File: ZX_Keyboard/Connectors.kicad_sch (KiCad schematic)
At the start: 18 parts

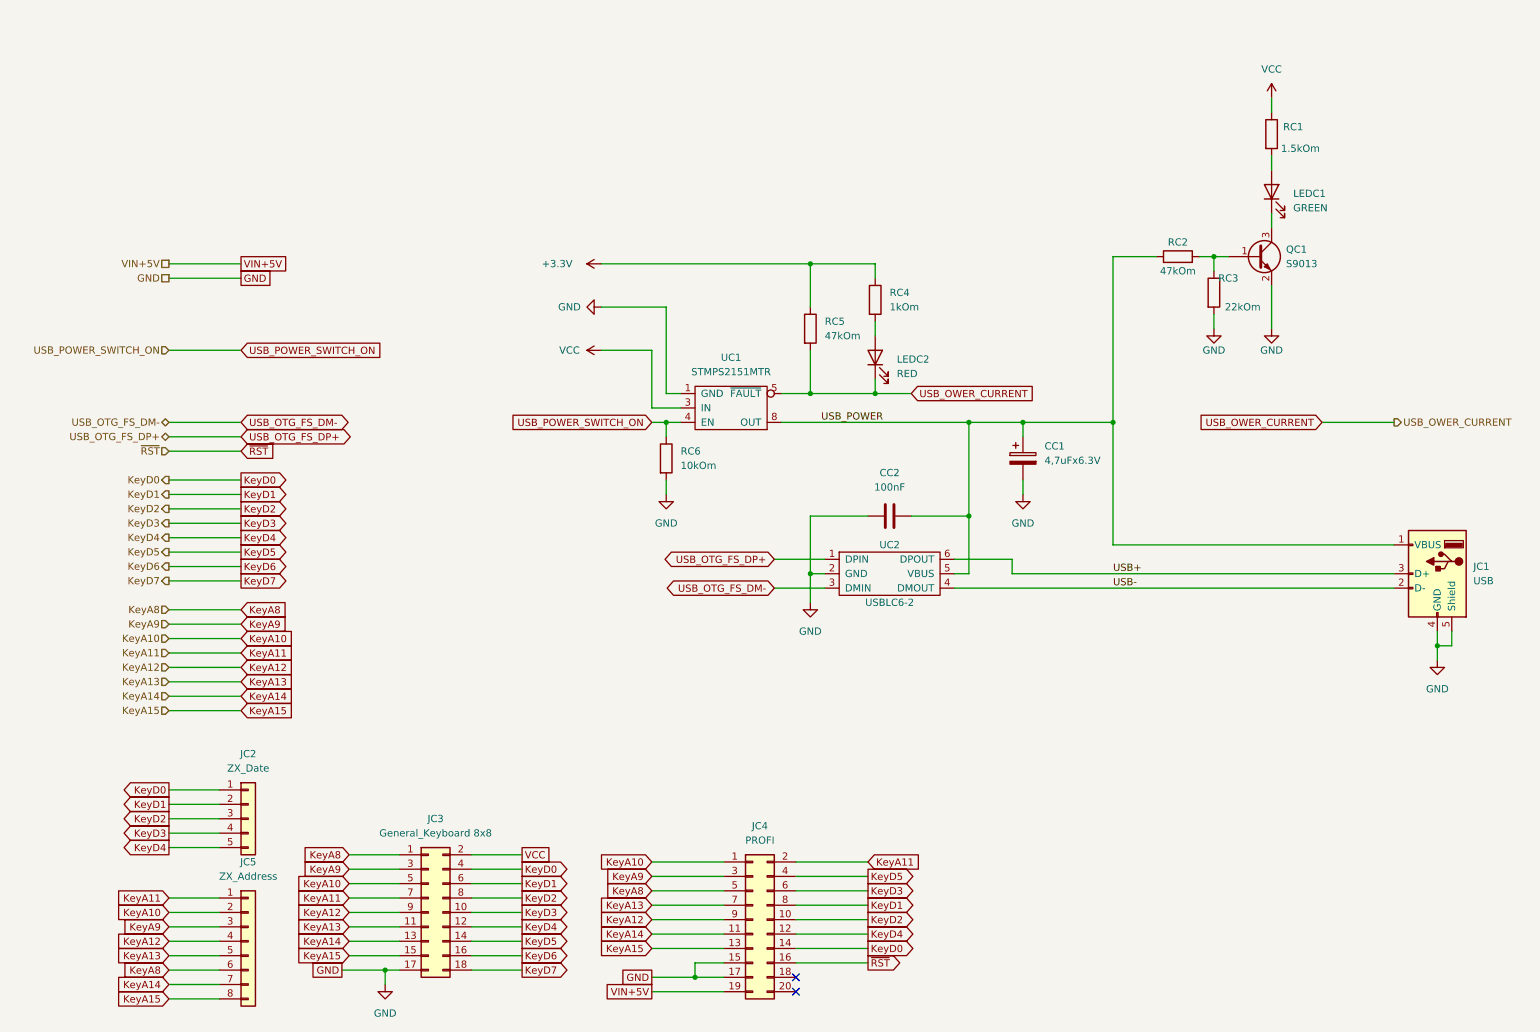
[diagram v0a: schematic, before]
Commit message: teracing and refactoring connectors
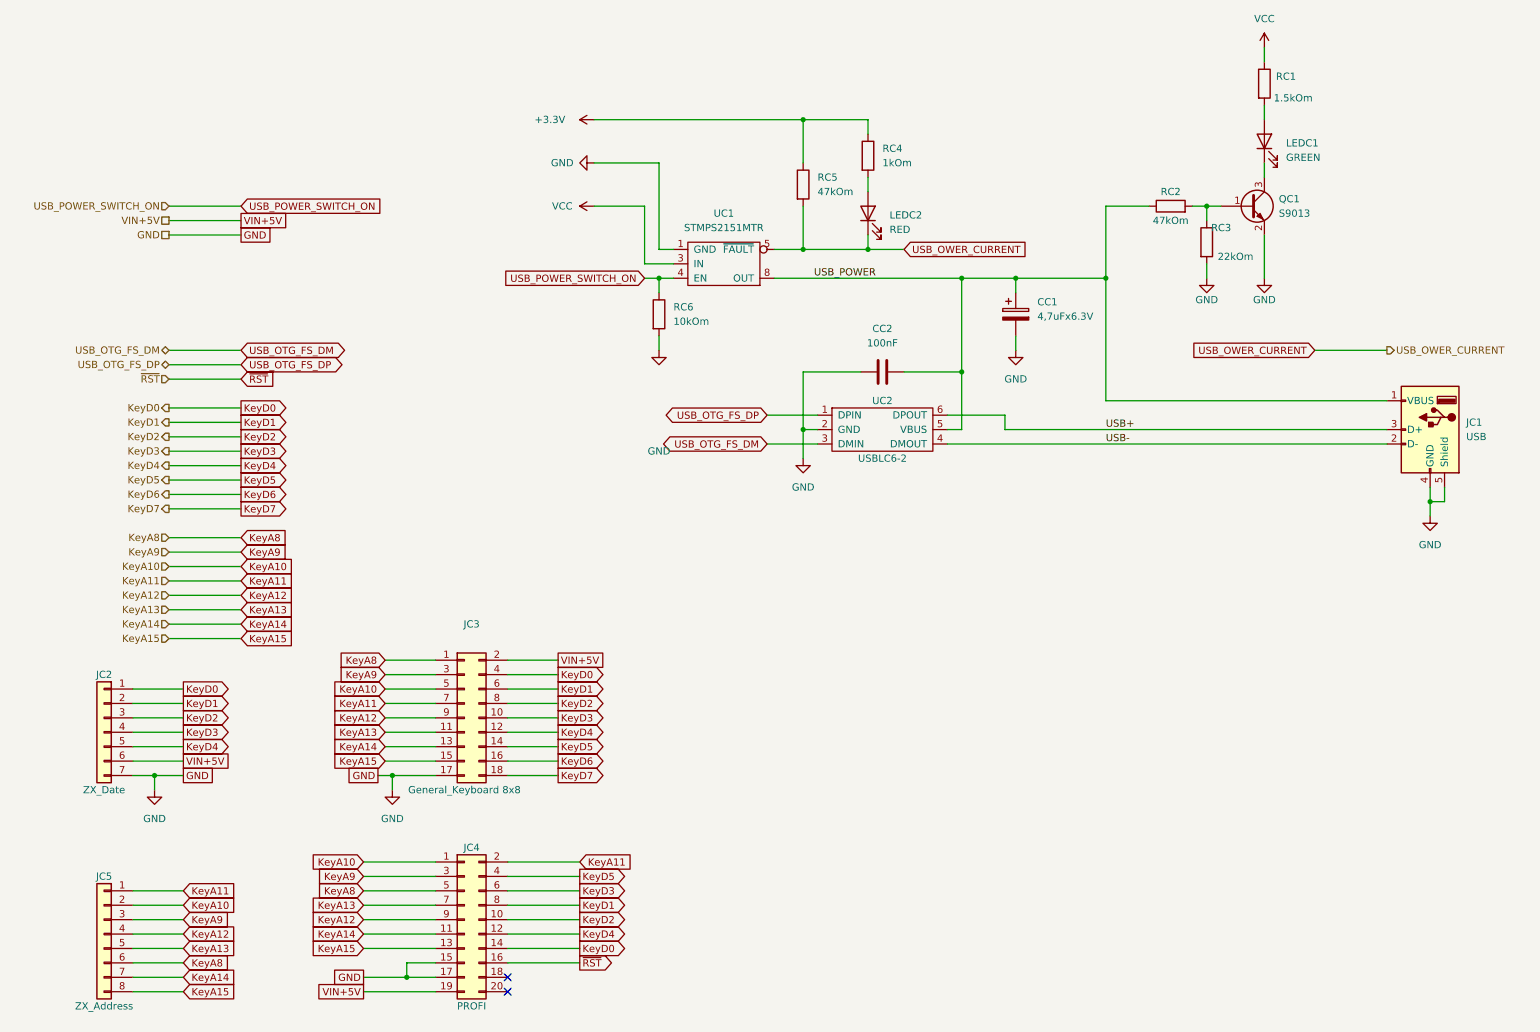
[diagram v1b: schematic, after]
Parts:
- removed JC2: ZX_Date, Connector_PinHeader_2.54mm:PinHeader_1x05_P2.54mm_Vertical, symbol Connector_Generic:Conn_01x05
- added JC2: ZX_Date, Connector_PinHeader_2.54mm:PinHeader_1x07_P2.54mm_Vertical, symbol Connector_Generic:Conn_01x07
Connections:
- net GND: now also JC2.7 (Pin_7)
- net IN: no longer JC3.2 (Pin_2)
- net KeyD0: now also JC2.1 (Pin_1)
- net KeyD1: now also JC2.2 (Pin_2)
- net KeyD2: now also JC2.3 (Pin_3)
- net KeyD3: now also JC2.4 (Pin_4)
- net KeyD4: now also JC2.5 (Pin_5)
- net VIN+5V: now also JC3.2 (Pin_2), JC2.6 (Pin_6)
- net USB_OTG_FS_DM- renamed USB_OTG_FS_DM
- net USB_OTG_FS_DP+ renamed USB_OTG_FS_DP
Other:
- moved on the sheet: CC1, CC2, JC1, JC3, JC4, JC5, LEDC1, LEDC2, QC1, RC1, RC2, RC3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
